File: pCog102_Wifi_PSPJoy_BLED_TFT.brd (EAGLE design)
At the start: 48 x 28 mm, 45 parts

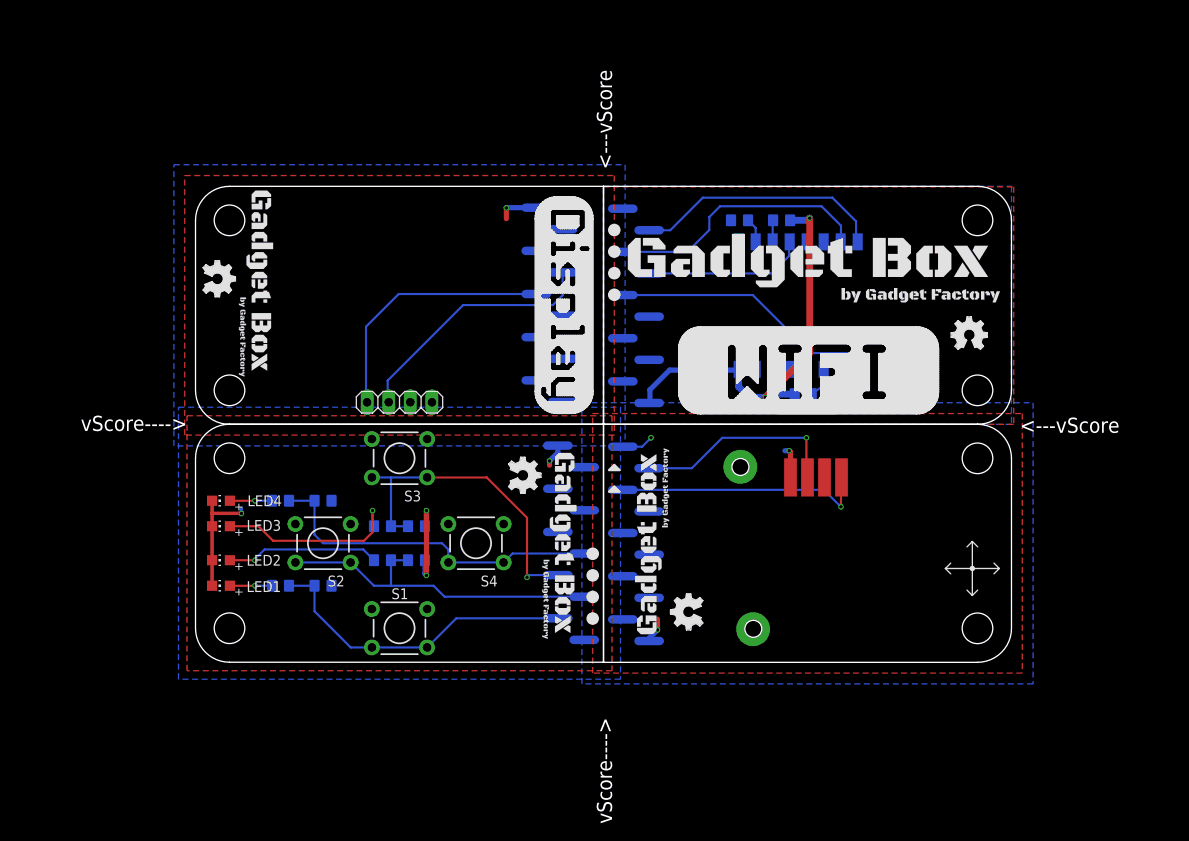
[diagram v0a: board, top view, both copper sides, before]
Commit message: All the 2.0 updates
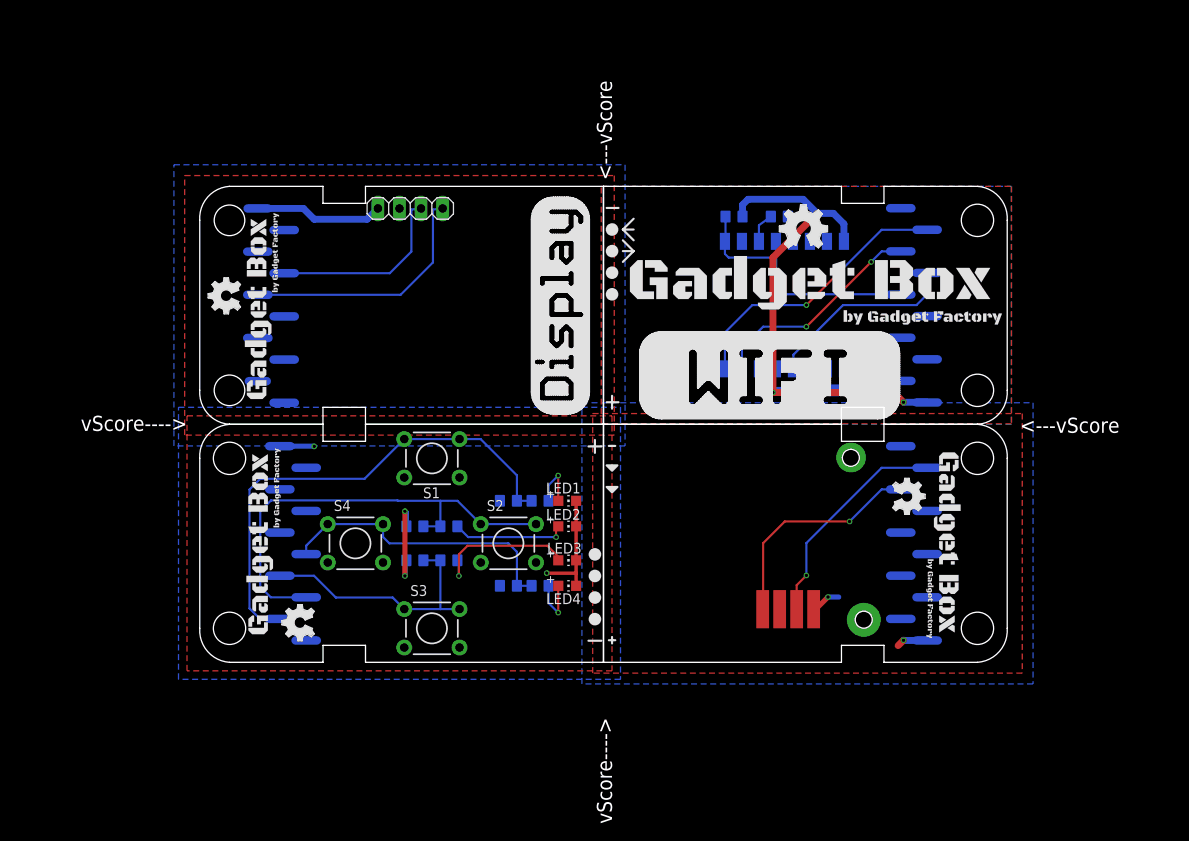
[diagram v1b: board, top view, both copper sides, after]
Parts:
- ECOG2: value ECOG_GENERAL_ROWECOG_GENERAL_SMD -> ECOG_BUSES_ROWECOG_BUSES_SMD; device eCogs:ECOG_GENERAL_SMD -> eCogs:ECOG_BUSES_SMD
- ECOG3: value ECOG_BUSES_ROWECOG_BUSES_SMD -> ECOG_GENERAL_ROWECOG_GENERAL_SMD; device eCogs:ECOG_BUSES_SMD -> eCogs:ECOG_GENERAL_SMD
- R1, R3: value 10K -> 390
- R11, R9: value 390 -> 10K
- U$1: device GadgetFactory:GADGETBOX_TEXT -> eCogs:LEGEND_DIO
- U$10, U$12, U$5: device eCogs:LEGEND_DIO -> GadgetFactory:GADGETBOX_SMALL
- U$11: device eCogs:LEGEND_DIO -> ohw-logo:OSHW_FILLX150_NOTEXT
- U$13: device GadgetFactory:GADGETBOX_SMALL -> ohw-logo:OSHW_FILLX150_NOTEXT
- U$14: device GadgetFactory:GADGETBOX_SMALL -> GadgetFactory:GADGETBOX_TEXT
- U$15: device GadgetFactory:GADGETBOX_SMALL -> eCogs:LEGEND_DIO
- U$16, U$17, U$18: device ohw-logo:OSHW_FILLX150_NOTEXT -> eCogs:LEGEND_DIO
- U$19: device ohw-logo:OSHW_FILLX150_NOTEXT -> ohw-logo:OSHW_FILLX200_NOTEXT
- U$6: value JOYSTICK-PSP1000 -> (none); device SparkFun:JOYSTICK-PSP1000 -> ohw-logo:OSHW_FILLX150_NOTEXT
- U$7: value (none) -> JOYSTICK-PSP1000; device eCogs:LEGEND_ANALOG -> SparkFun:JOYSTICK-PSP1000
- U$9: device eCogs:LEGEND_DIO -> eCogs:LEGEND_ANALOG
- moved R12 63.2 mm to (68.7, 52.4), turned to 180 degrees
- moved R11 63.0 mm to (63.4, 52.4), turned to 180 degrees
- moved U$6 60.1 mm to (14.0, 2.54), turned to 90 degrees
- moved ECOG 55.6 mm to (0.00, 0.00)
- moved ECOG1 55.6 mm to (96.0, 28.0), turned to 180 degrees
- moved R10 52.7 mm to (76.2, 32.0)
- moved R9 51.8 mm to (71.2, 32.0)
- moved U$5 50.9 mm to (7.62, 14.0), turned to 90 degrees
- moved R3 49.5 mm to (29.8, 16.0), turned to 180 degrees
- moved U$12 48.8 mm to (7.44, 41.6), turned to 90 degrees
- moved U$18 48.3 mm to (49.0, 50.9), turned to 180 degrees
- moved R4 48.3 mm to (25.8, 16.0), turned to 180 degrees
- moved U$16 48.1 mm to (49.0, 45.8), turned to 180 degrees
- moved ECOG2 48.0 mm to (-0.01, 28.0), turned to 0 degrees
- moved ECOG3 48.0 mm to (96.0, 56.0)
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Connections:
- removed net N$5: R4.1, X1.3
- removed net N$6: LED1.A, R5.2
- removed net RX: ECOG.G1, X1.15
- removed net TX: ECOG.G0, X1.16
- new net N$1: LED1.A, R1.2
- new net N$2: LED2.A, R3.2
- new net RX/MOSI: ECOG3.G1, X1.15
- new net TX/MISO: ECOG3.G0, X1.16
- net 1: now also ECOG.G0, R1.1, R2.2; no longer ECOG2.G0, R5.1, R6.2
- net 2: now also ECOG.G1, R3.1, R4.2; no longer ECOG2.G1, R7.1, R8.2
- net 3: now also ECOG.G2, R5.1, R6.2; no longer ECOG2.G2, R10.2, R9.1
- net 3V3: now also R11.2, R12.2, R9.2, U$7.VCC; no longer R1.2, R3.2, R4.2, U$6.VCC
- net 4: now also ECOG.G3, R7.1, R8.2; no longer ECOG2.G3, R11.1, R12.2
- net GND: now also R4.1, U$7.GND; no longer R12.1, U$6.GND
- net GPIO0/BOOTLOAD: now also ECOG3.G2; no longer ECOG.G2
- net HORIZONTAL: now also U$7.X; no longer U$6.X
- net N$10: now also R10.2, X1.10; no longer ECOG3.I2C-SDA, JP1.4
- net N$11: now also R12.1, X1.3; no longer ECOG3.I2C-SCL, JP1.3
- net N$3: now also LED3.A, R5.2; no longer R1.1, X1.11
- net N$4: now also LED4.A, R7.2; no longer R2.2, X1.10
- net N$7: now also ECOG2.I2C-SDA, JP1.4; no longer LED2.A, R7.2
- net N$8: now also ECOG2.I2C-SCL, JP1.3; no longer LED3.A, R9.2
- net N$9: now also R9.1, X1.11; no longer LED4.A, R11.2
- net RESET: now also ECOG3.G3, R11.1; no longer ECOG.G3, R3.1
- net VERTICAL: now also U$7.Y; no longer U$6.Y
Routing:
- net TX/MISO: track 0.00 -> 33.3 mm, vias 0 -> 2
- net RX: track 31.6 -> 0.00 mm
- net TX: track 29.6 -> 0.00 mm
- net N$10: track 30.6 -> 2.90 mm
- net N$11: track 30.0 -> 3.63 mm
- net RX/MOSI: track 0.00 -> 25.9 mm, vias 0 -> 2
- net 1: track 37.8 -> 58.5 mm
- net 3V3: track 69.6 -> 87.8 mm
- net N$3: track 2.56 -> 18.2 mm, vias 0 -> 1
- net N$2: track 0.00 -> 13.5 mm
- net 2: track 40.6 -> 53.9 mm
- net N$7: track 18.1 -> 29.5 mm, vias 1 -> 0
- net 3: track 38.7 -> 30.5 mm, vias 1 -> 0
- net 4: track 41.4 -> 34.8 mm
- net N$1: track 0.00 -> 6.41 mm
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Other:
- board size 48 x 28 mm -> 47.5 x 28 mm
- board text added: "0"
- board text added: "1"
- board text added: "2"
- board text added: "3"
- board text added: "Horizontal"
- board text added: "L/S1"
- board text added: "L/S2"
- board text added: "L/S3"
- board text added: "L/S4"
- board text added: "RX/MOSI"
- board text added: "TX/MISO"
- board text added: "Vert"
- board text added: "ecog100 v2.0"
- board text added: "ecog101 v2.0"
- board text added: "ecog104 v2.0"
- board text added: "ecog106 v2.0"
- board text removed: "Horizontal<"
- board text removed: "P1<>"
- board text removed: "P2<>"
- board text removed: "P3<>"
- board text removed: "P4<>"
- board text removed: "RX>"
- board text removed: "TX<"
- board text removed: "Vertical<"
- board text removed: "ecog100 v1.1"
- board text removed: "ecog101 v1.1"
- board text removed: "ecog104 v1.0"
- board text removed: "ecog106 v1.1"
